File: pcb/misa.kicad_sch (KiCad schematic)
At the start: 81 parts, among them J1 PLD JTAG, J2 CF CARD, J3 44 PIN IDE, J4 UART, J5 Headphones, K1 G5V-2, Q1 NPN, SW1 Reset, U1 MC68000P, U10 SST39SF040, U11 SST39SF040, U12 WizFi360, U13 AS6C4008-55PCN, U14 AS6C4008-55PCN, U15 YM2151, U16 TDA2822M, U17 YM3012, U2 ATF1508ASx-xxJx84, U3 NE555P, U4 74LS05, U5 KNY320240B, U6 74HC74, U7 TL074, U8 18650 Holder, U9 16550, Y1 16 MHz, Y2 1.8432 MHz, Y3 3.579545 MHz

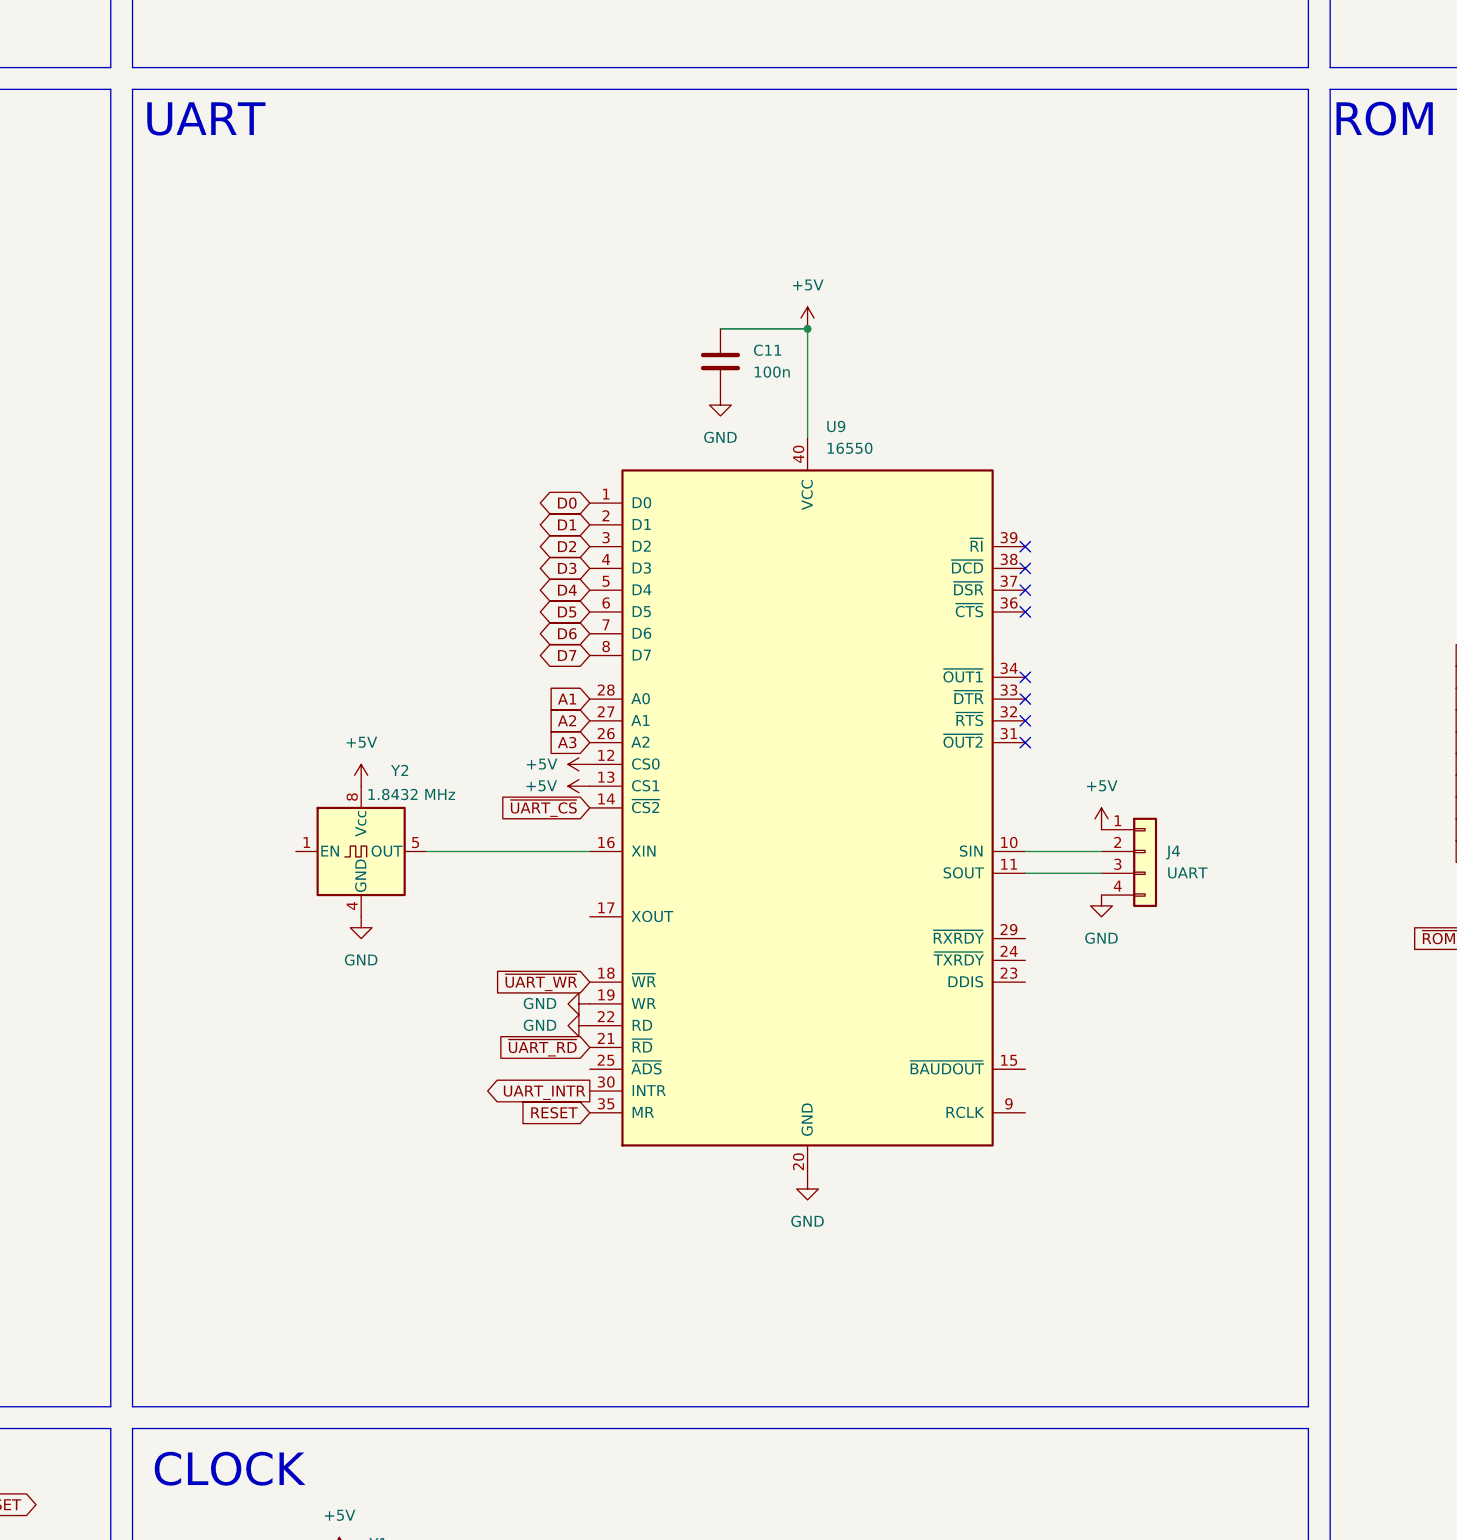
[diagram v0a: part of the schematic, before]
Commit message: stuff
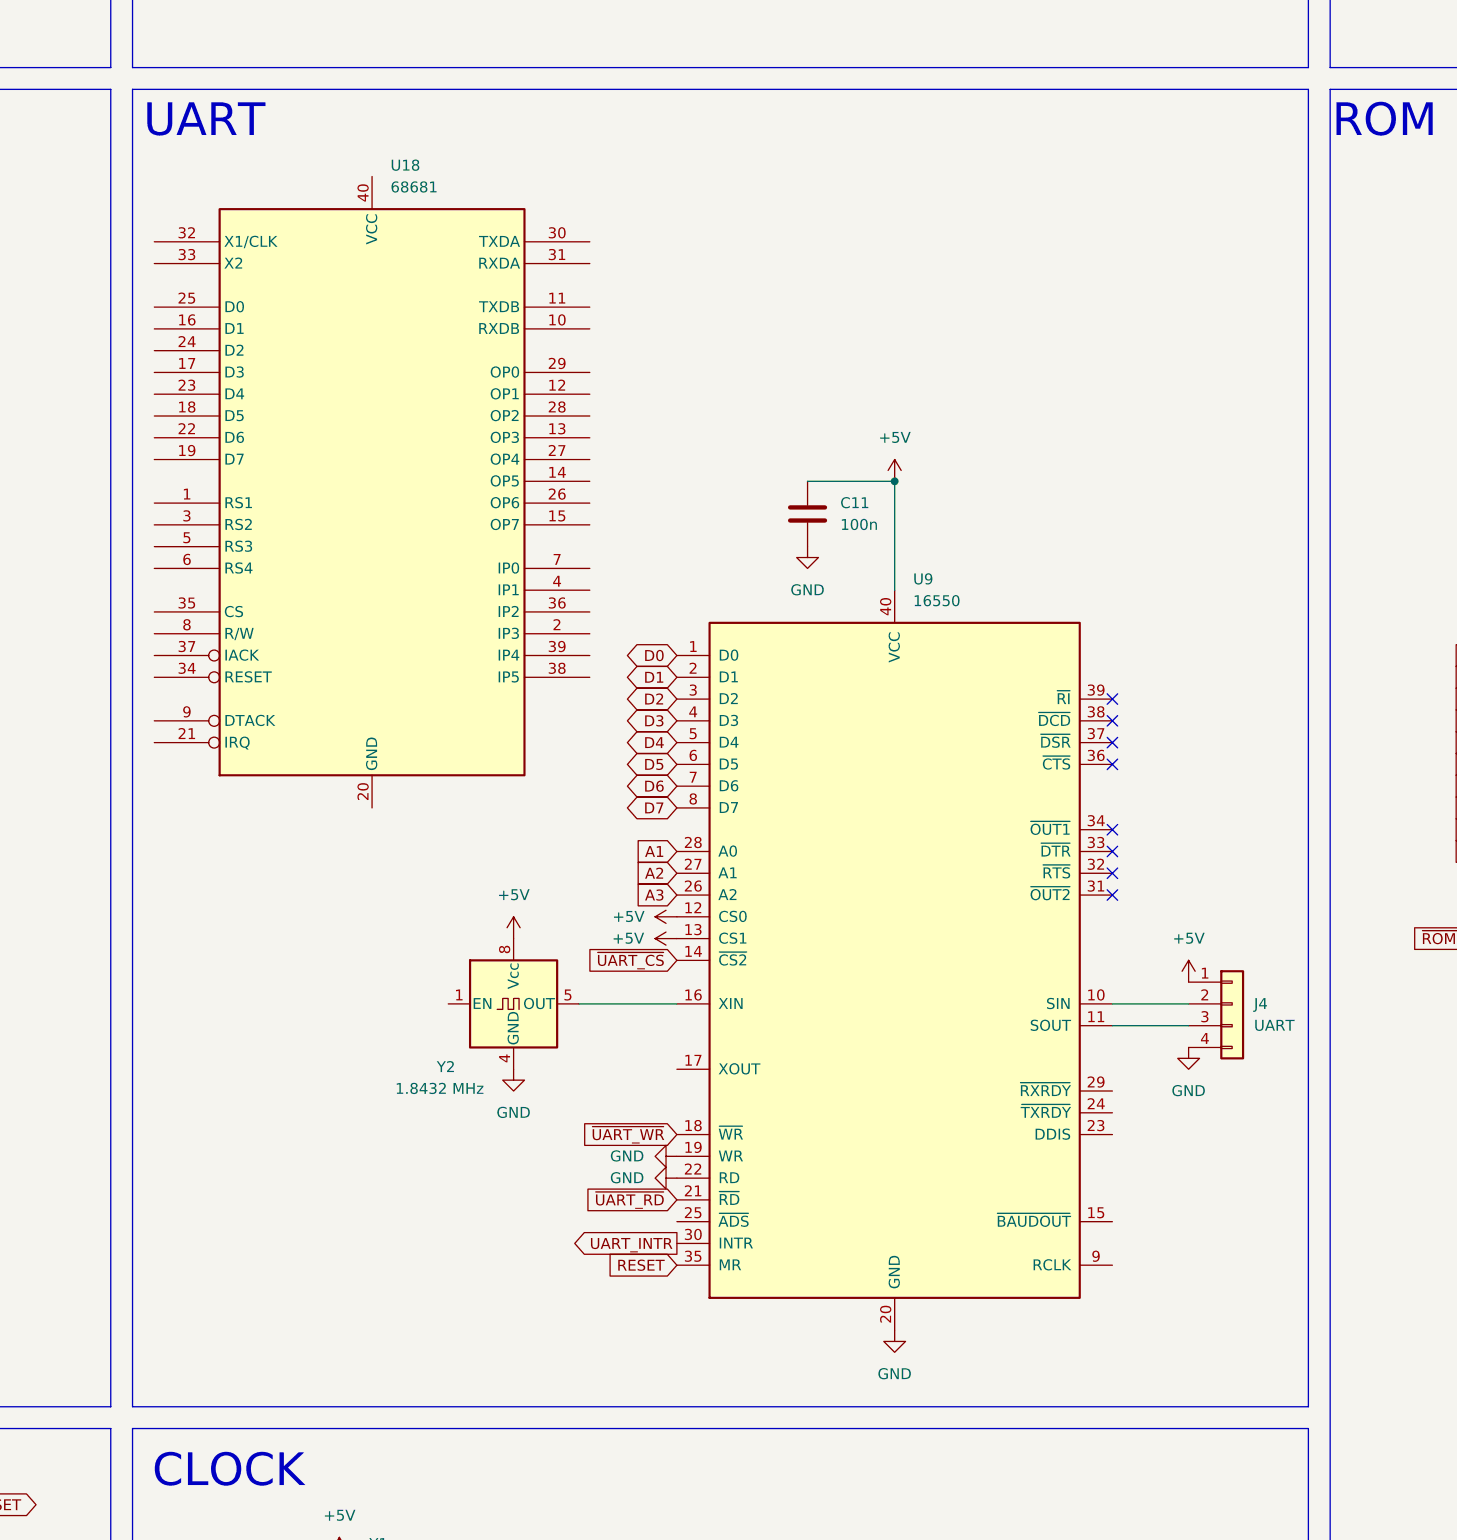
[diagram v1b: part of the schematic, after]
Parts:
- added U18: 68681, symbol Interface:68681
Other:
- moved on the sheet: C11, J4, U9, Y2

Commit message: stuff
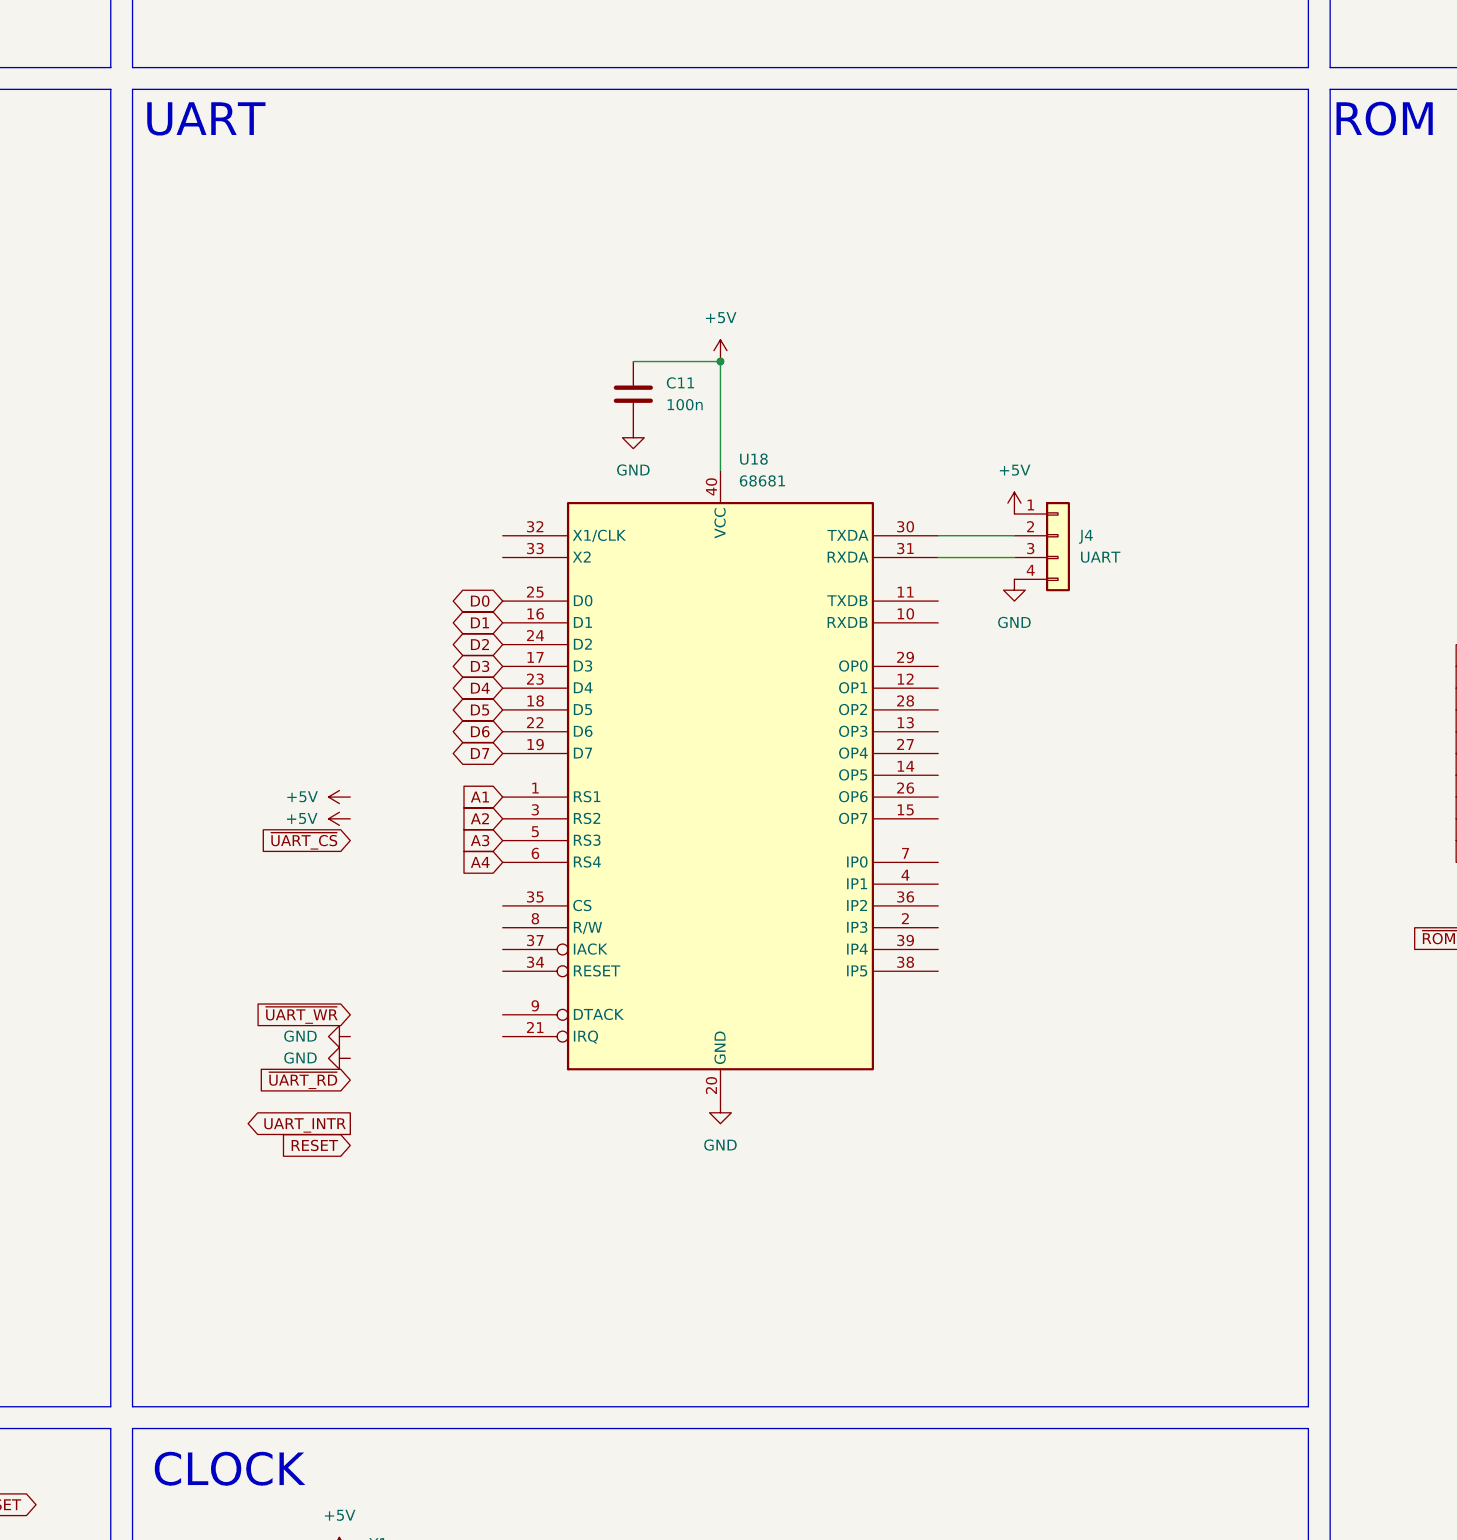
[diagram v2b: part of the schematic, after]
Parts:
- removed U9: 16550, Package_LCC:PLCC-44_THT-Socket, symbol Interface_UART:16550
- removed Y2: 1.8432 MHz, Oscillator:Oscillator_DIP-8, symbol Oscillator:CXO_DIP8
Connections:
- net +5V: now also U18.40 (VCC)
- net A1: now also U18.1 (RS1)
- net A2: now also U18.3 (RS2)
- net A3: now also U18.5 (RS3)
- net A4: now also U18.6 (RS4)
- net D0: now also U18.25 (D0)
- net D1: now also U18.16 (D1)
- net D2: now also U18.24 (D2)
- net D3: now also U18.17 (D3)
- net D4: now also U18.23 (D4)
- net D5: now also U18.18 (D5)
- net D6: now also U18.22 (D6)
- net D7: now also U18.19 (D7)
- net GND: now also U18.20 (GND)
- net at U18.30 (TXDA): now also J4.2 (Pin_2)
- net at U18.31 (RXDA): now also J4.3 (Pin_3)
- no-connect marks 20 -> 12
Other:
- moved on the sheet: C11, J4, U18
